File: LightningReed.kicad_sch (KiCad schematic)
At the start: 12 parts, among them P1 Conn_WallPlug

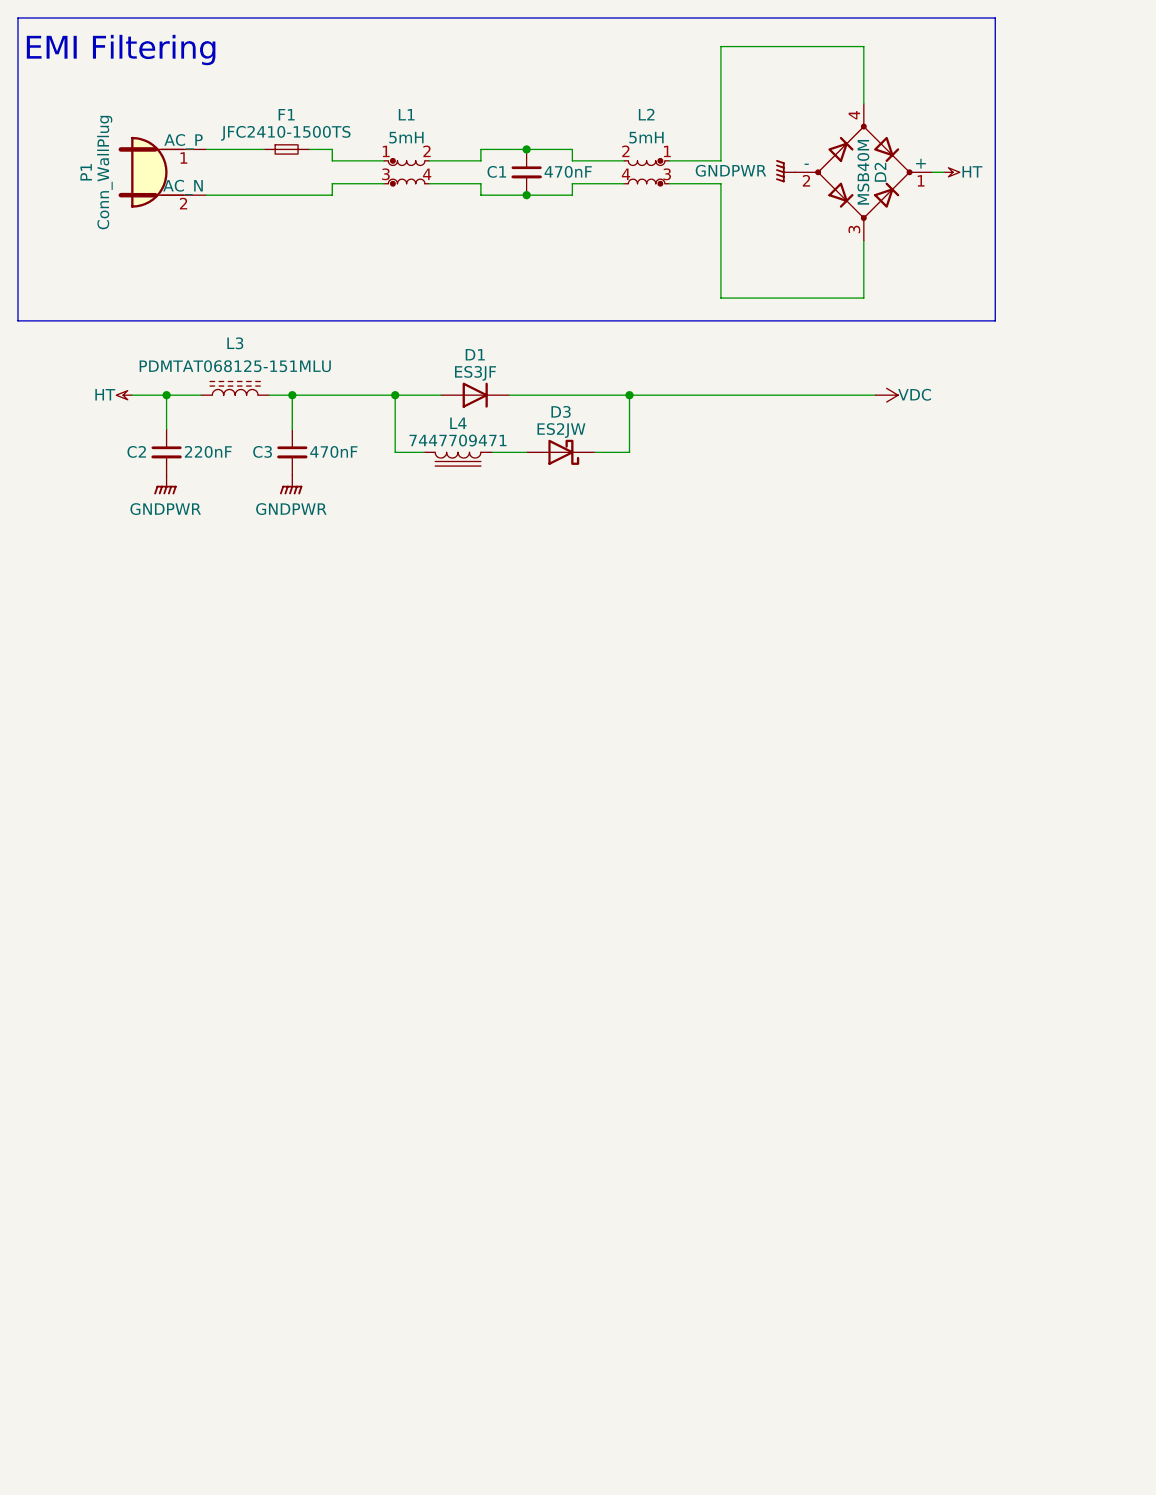
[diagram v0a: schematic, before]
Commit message: PFC
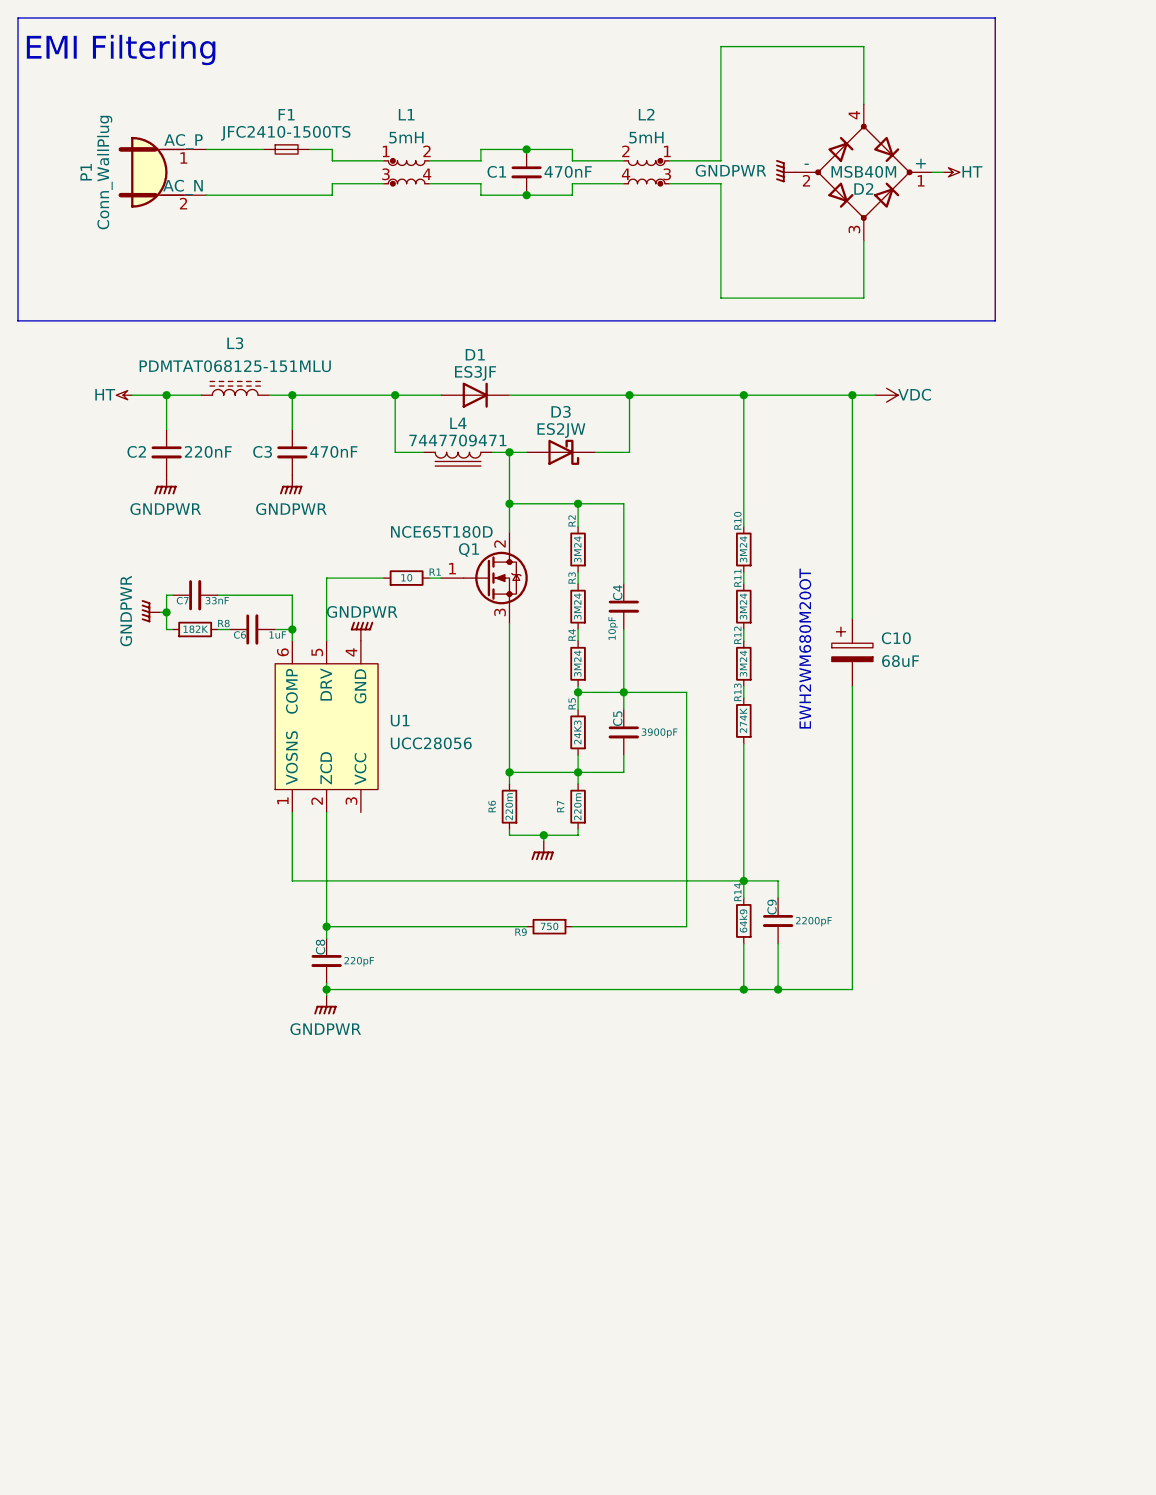
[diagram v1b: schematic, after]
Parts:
- added C10: 68uF, symbol Device:C_Polarized
- added C4: 10pF, symbol Device:C_Small
- added C5: 3900pF, symbol Device:C_Small
- added C6: 1uF, symbol Device:C_Small
- added C7: 33nF, symbol Device:C_Small
- added C8: 220pF, symbol Device:C_Small
- added C9: 2200pF, symbol Device:C_Small
- added Q1: NCE65T180D, symbol Device:Q_NMOS_GDS
- added R1: 10, symbol Device:R_Small
- added R10, R11, R12, R2, R3, R4: 3M24, symbol Device:R_Small
- added R13: 274K, symbol Device:R_Small
- added R14: 64k9, symbol Device:R_Small
- added R5: 24K3, symbol Device:R_Small
- added R6, R7: 220m, symbol Device:R_Small
- added R8: 182K, symbol Device:R_Small
- added R9: 750, symbol Device:R_Small
- added U1: UCC28056, symbol LightningReed:UCC28056
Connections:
- net GNDPWR: now also C10.2, C7.1, C8.2, C9.2, R14.1, R6.1, R7.1, R8.1, U1.4 (GND)
- net VDC: now also C10.1, R10.2
- net at D3.2 (A), L4.1: now also C4.1, Q1.2 (D), R2.2
- new net: R1.1, U1.5 (DRV)
- new net: Q1.1 (G), R1.2
- new net: R3.1, R4.2
- new net: R2.1, R3.2
- new net: C5.2, Q1.3 (S), R5.1, R6.2, R7.2
- new net: C4.2, C5.1, R4.1, R5.2, R9.1
- new net: R12.1, R13.2
- new net: R11.1, R12.2
- new net: C6.1, R8.2
- new net: C6.2, C7.2, U1.6 (COMP)
- new net: C9.1, R13.1, R14.2, U1.1 (VOSNS)
- new net: C8.1, R9.2, U1.2 (ZCD)
- new net: R10.1, R11.2
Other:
- note added: "EWH2WM680M20OT"

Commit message: brown out circuit
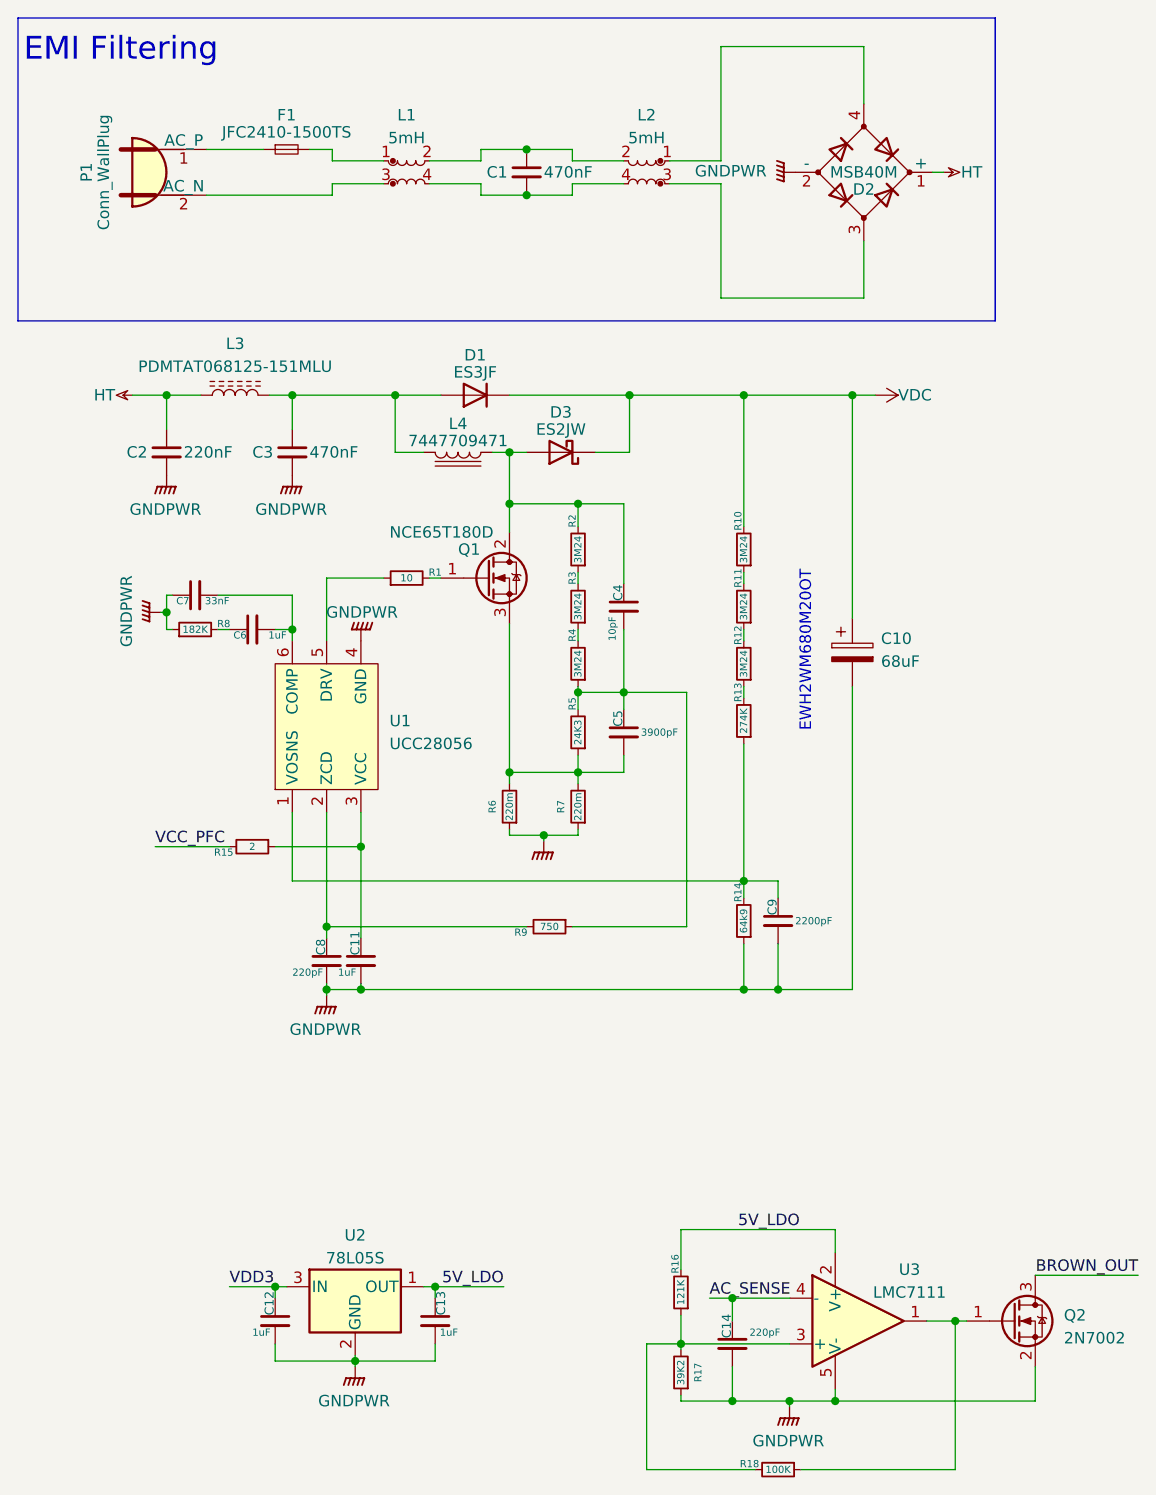
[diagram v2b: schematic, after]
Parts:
- added C11, C12, C13: 1uF, symbol Device:C_Small
- added C14: 220pF, symbol Device:C_Small
- added Q2: 2N7002, Package_TO_SOT_SMD:SOT-23, symbol Transistor_FET:2N7002
- added R15: 2, symbol Device:R_Small
- added R16: 121K, symbol Device:R_Small
- added R17: 39K2, symbol Device:R_Small
- added R18: 100K, symbol Device:R_Small
- added U2: 78L05S, Package_TO_SOT_SMD:SOT-89-3, symbol Regulator_Linear:L78L05_SOT89
- added U3: LMC7111, symbol LightningReed:LMC7111
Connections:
- net GNDPWR: now also C11.2, C12.2, C13.2, C14.2, Q2.2 (S), R17.1, U2.2 (GND), U3.5 (V-)
- net at U1.3 (VCC): now also C11.1, R15.1
- new net: Q2.1 (G), R18.1, U3.1
- new net: R16.1, R17.2, R18.2, U3.3 (+)
- new net 5V_LDO: C13.1, R16.2, U2.1 (OUT), U3.2 (V+)
- new net AC_SENSE: C14.1, U3.4 (-)
- new net BROWN_OUT: Q2.3 (D)
- new net VCC_PFC: R15.2
- new net VDD3: C12.1, U2.3 (IN)
